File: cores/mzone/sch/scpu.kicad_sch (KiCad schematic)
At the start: 33 parts, among them X1 14.318MHZ

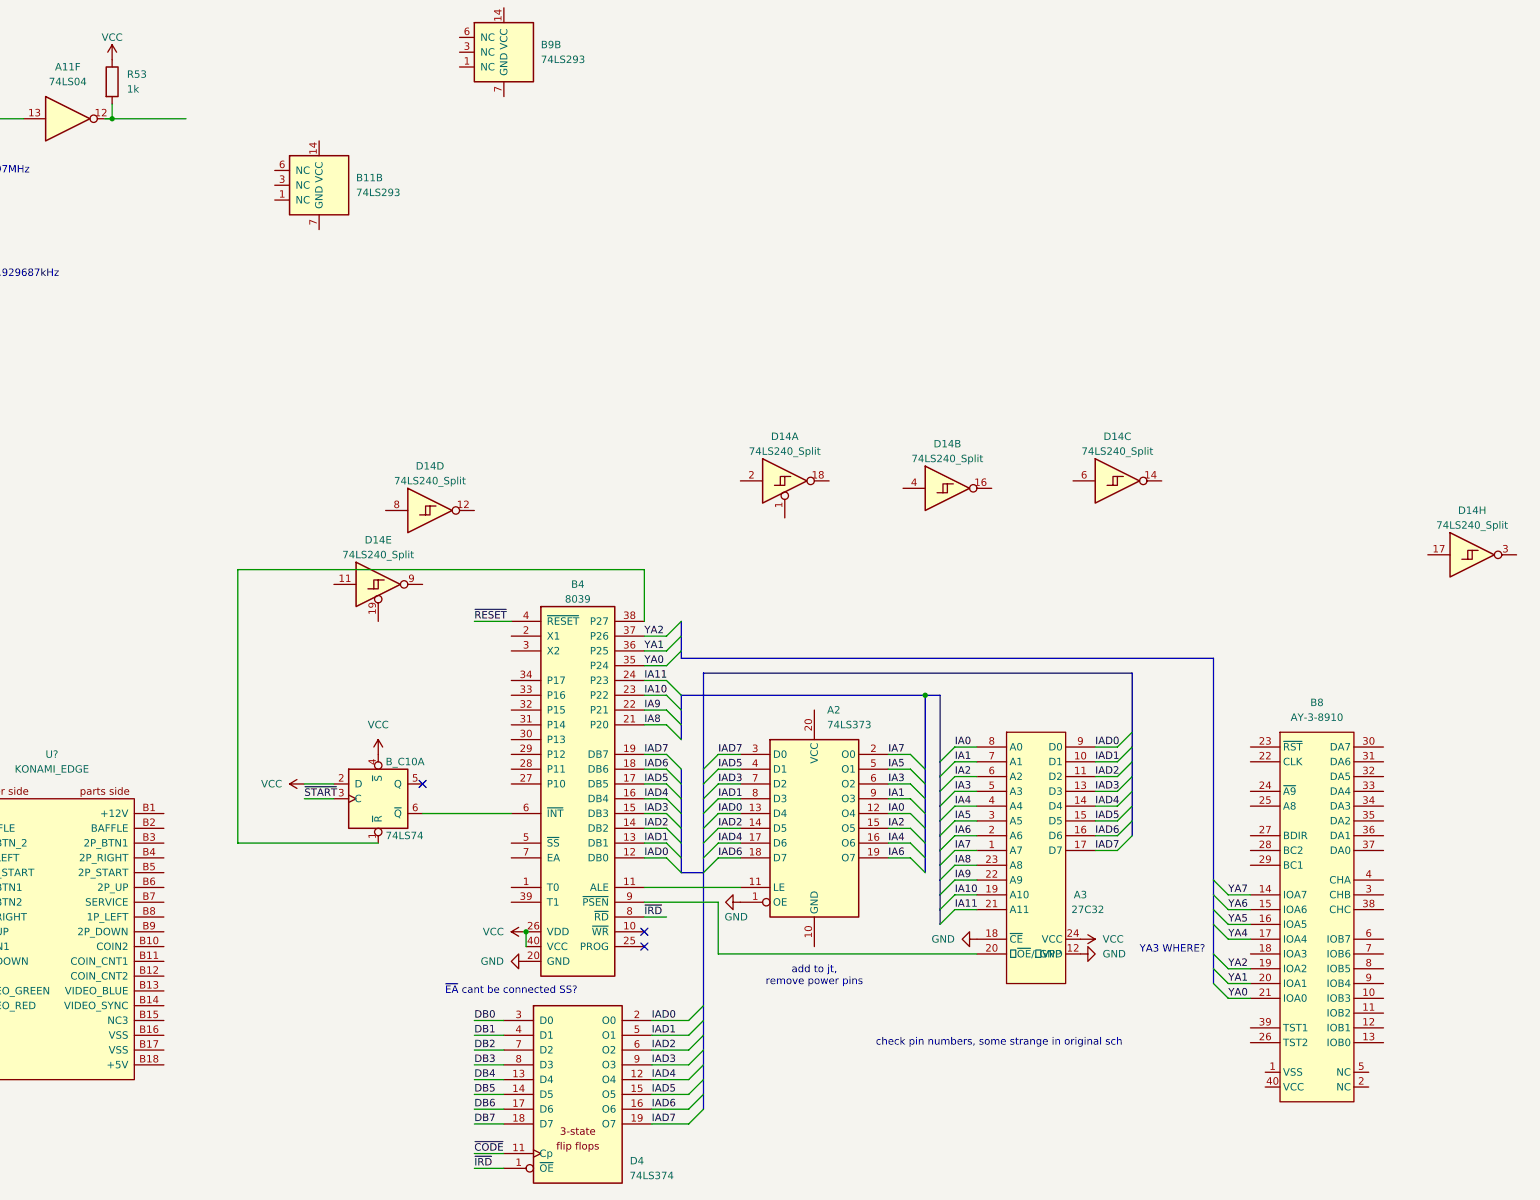
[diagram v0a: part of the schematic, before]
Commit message: mzone core sch
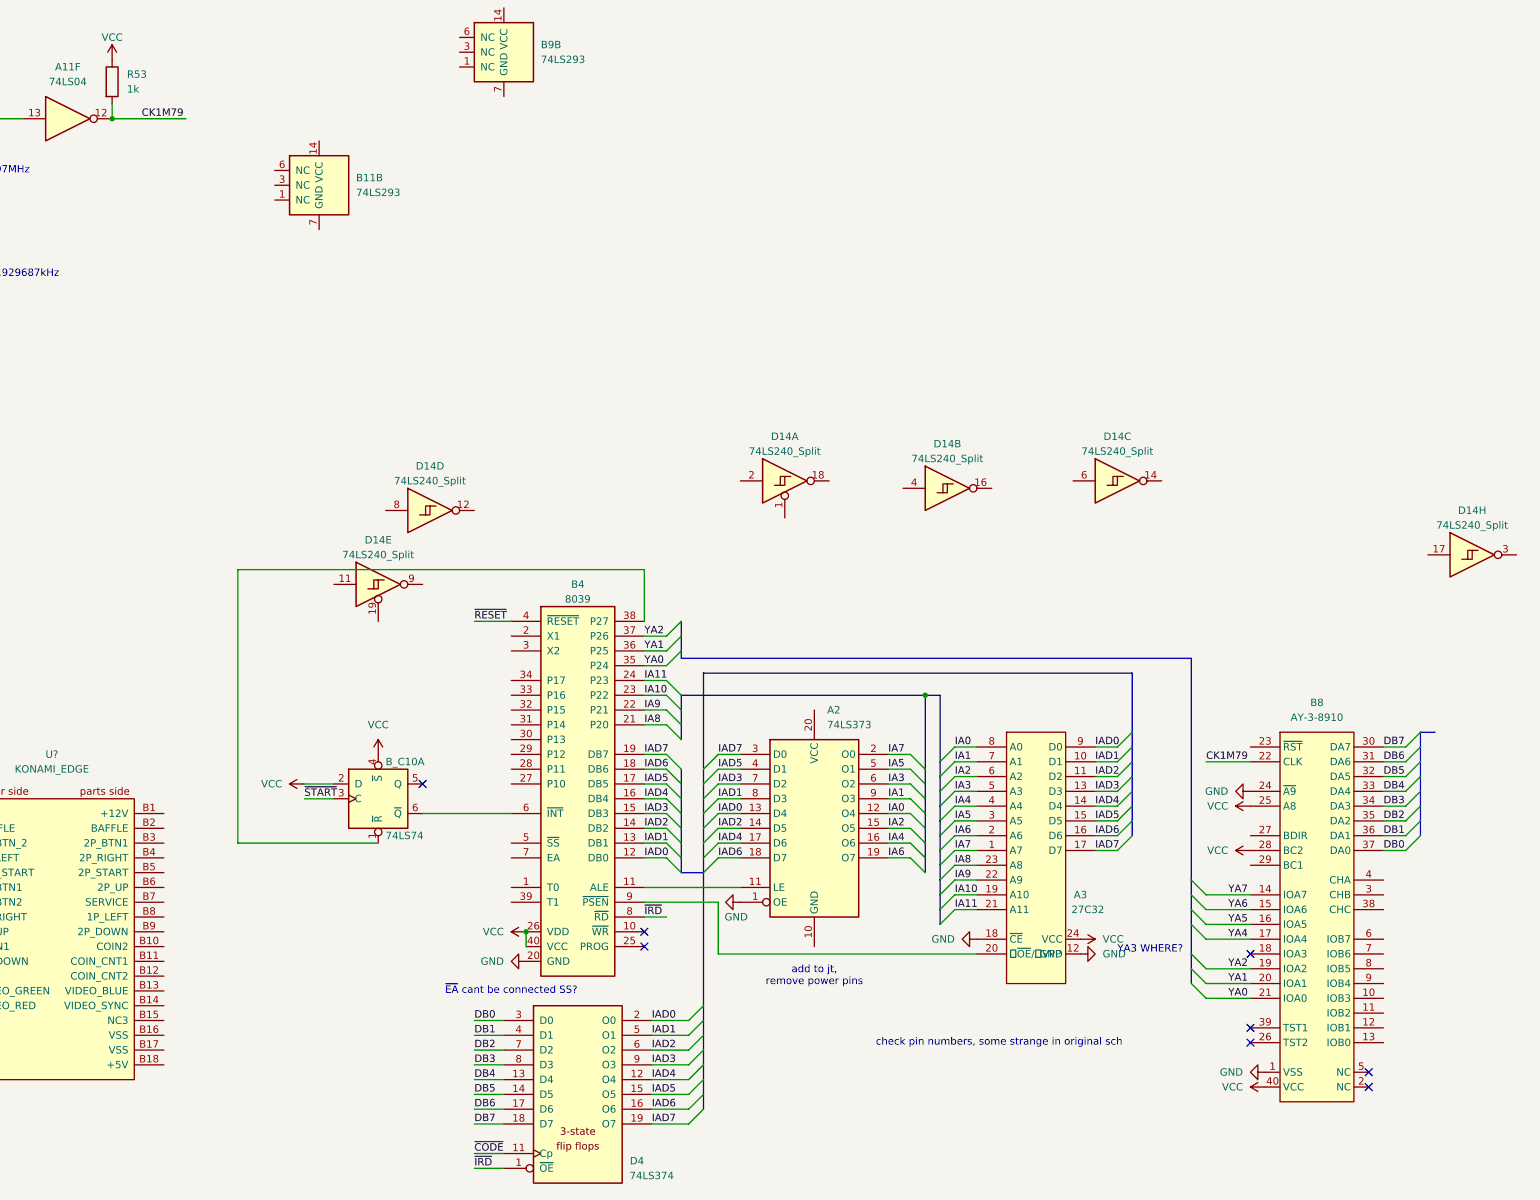
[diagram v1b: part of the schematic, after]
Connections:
- net DB0: now also B8.37 (DA0)
- net DB1: now also B8.36 (DA1)
- net DB2: now also B8.35 (DA2)
- net DB3: now also B8.34 (DA3)
- net DB4: now also B8.33 (DA4)
- net DB5: now also B8.32 (DA5)
- net DB6: now also B8.31 (DA6)
- net DB7: now also B8.30 (DA7)
- net GND: now also B8.1 (VSS), B8.24 (~{A9})
- net VCC: now also B8.25 (A8), B8.28 (BC2), B8.40 (VCC)
- net CK1M79: now reaches B8.22 (CLK)
- net CK1M79: now also A11.12, R53.2
- no-connect marks 6 -> 11
